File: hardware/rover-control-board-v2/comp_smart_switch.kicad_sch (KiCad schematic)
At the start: 26 parts, among them Q3 Q_NMOS_DGS, Q4 Q_PMOS_DGS, U2 BTH50015

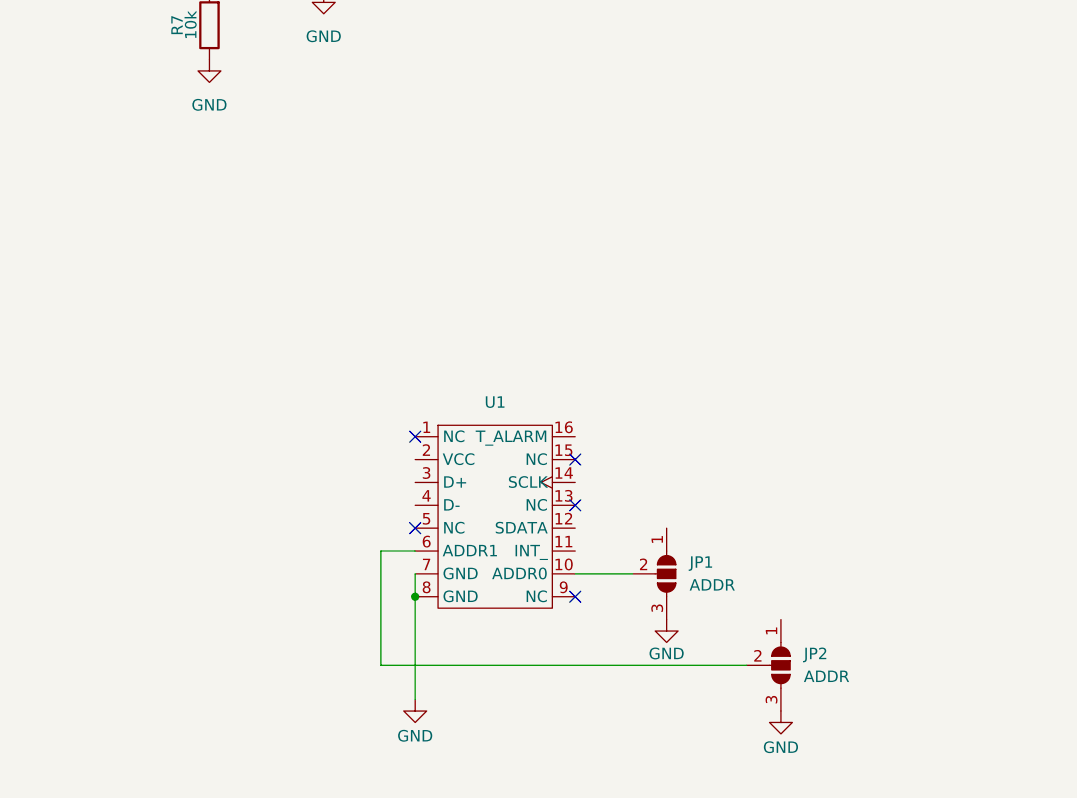
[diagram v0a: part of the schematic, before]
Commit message: progress
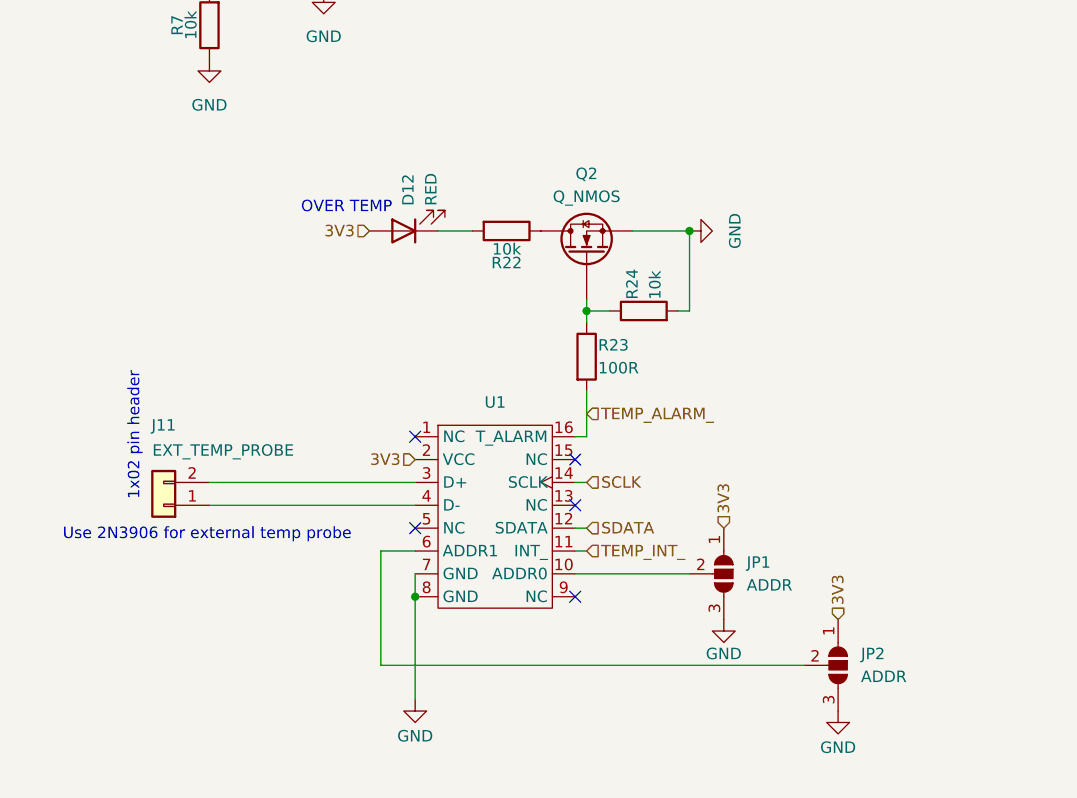
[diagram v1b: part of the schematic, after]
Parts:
- added D12: RED, symbol Device:LED
- added J11: EXT_TEMP_PROBE, symbol Connector_Generic:Conn_01x02
- added Q2: Q_NMOS, symbol Device:Q_NMOS
- added R22, R24: 10k, symbol Device:R
- added R23: 100R, symbol Device:R
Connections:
- net GND: now also Q2.S, R24.2
- net 3V3: now reaches JP2.1 (A)
- net 3V3: now also JP1.1 (A), U1.2 (VCC), D12.2 (A)
- net TEMP_INT_: now reaches U1.11 (INT_)
- net SDATA: now reaches U1.12 (SDATA)
- net SCLK: now reaches U1.14 (SCLK)
- net TEMP_ALARM_: now reaches U1.16 (T_ALARM)
- net TEMP_ALARM_: now also R23.2
- net at U1.3 (D+): now also J11.2 (Pin_2)
- net at U1.4 (D-): now also J11.1 (Pin_1)
- new net: D12.1 (K), R22.2
- new net: Q2.D, R22.1
- new net: Q2.G, R23.1, R24.1
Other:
- note added: "1x02 pin header"
- note added: "OVER TEMP"
- note added: "Use 2N3906 for external temp probe"
- moved on the sheet: JP1, JP2
